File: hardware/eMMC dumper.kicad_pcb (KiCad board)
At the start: 2 copper layers, 67 x 43.2 mm, 52 parts, among them J1 Micro_SD_Card, J2 USB_B_Micro, J3 Conn_01x04, U1 F1C100s, U2 AMS1117-3.3, U3 TLV75512PDBV (WL9193S5-12), U4 EMMC04G-M627-A01

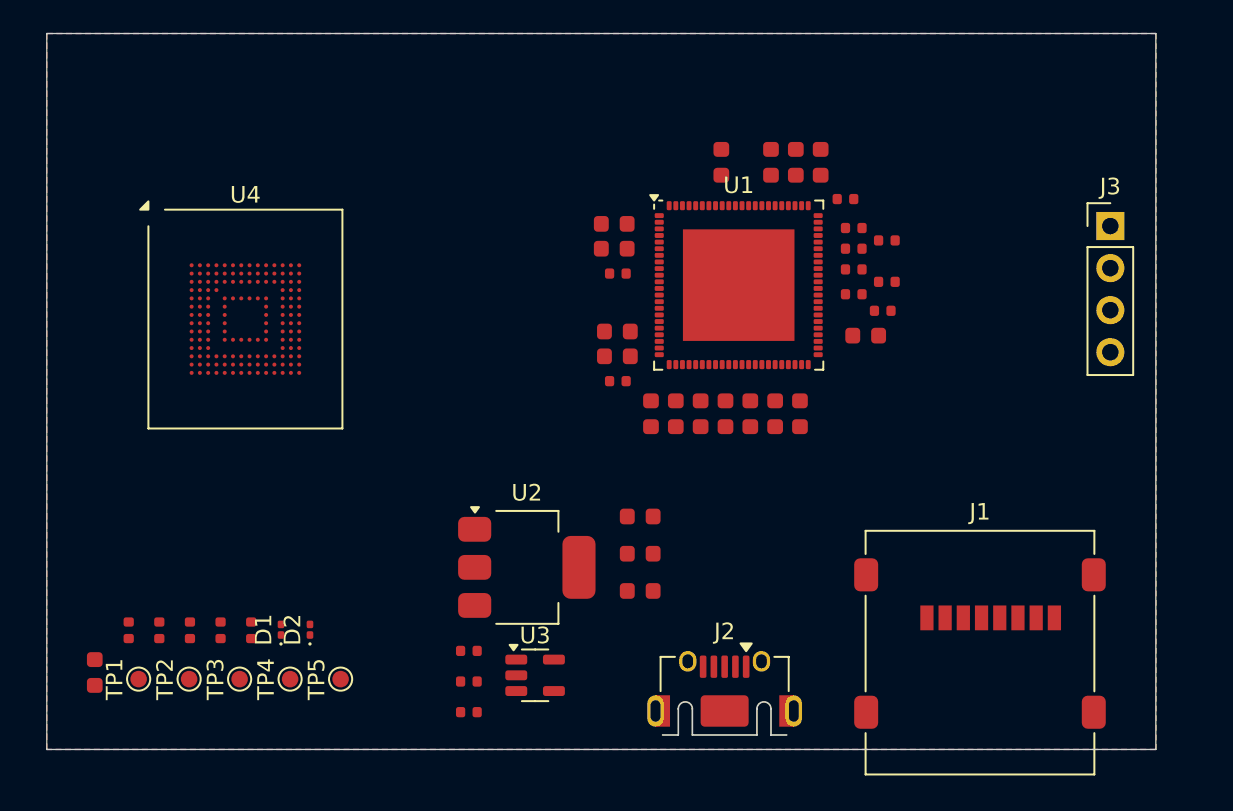
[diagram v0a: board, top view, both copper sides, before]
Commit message: PCB major changes
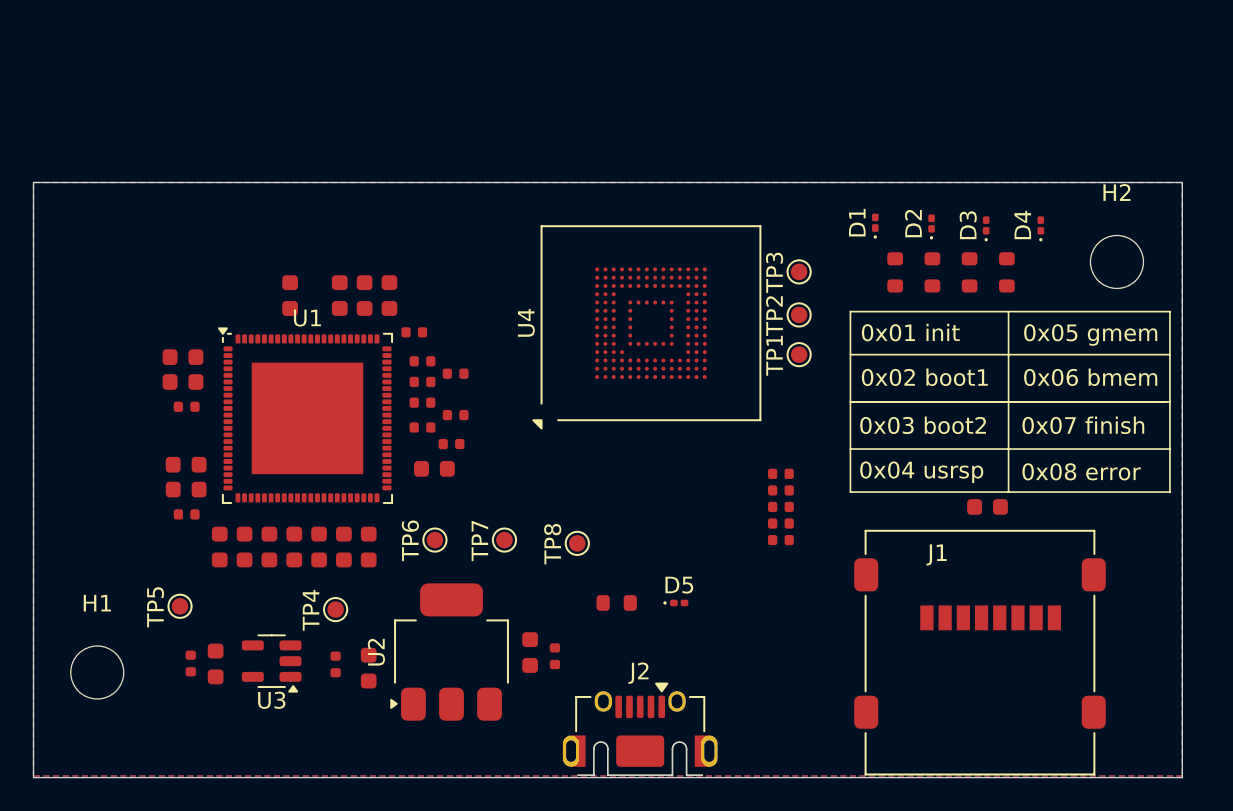
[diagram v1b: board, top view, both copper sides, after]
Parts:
- removed J3: Conn_01x04, Connector_PinHeader_2.54mm:PinHeader_1x04_P2.54mm_Vertical
- added D3: LED, LED_SMD:LED_0201_0603Metric, F.Cu at (182.5, 93.6)
- added D4: LED, LED_SMD:LED_0201_0603Metric, F.Cu at (185.8, 93.6)
- added D5: LED, LED_SMD:LED_0201_0603Metric, F.Cu at (164.0, 116.4)
- added H1: MountingHole, MountingHole:MountingHole_3.2mm_M3, F.Cu at (128.8, 120.6)
- added H2: MountingHole, MountingHole:MountingHole_3.2mm_M3, F.Cu at (190.4, 95.8)
- added R13: 1kΩ, PCM_JLCPCB:R_0603, F.Cu at (177.0, 96.4)
- added R14: 1kΩ, PCM_JLCPCB:R_0603, F.Cu at (179.2, 96.4)
- added R15: 1kΩ, PCM_JLCPCB:R_0603, F.Cu at (181.5, 96.4)
- added R16: 1kΩ, PCM_JLCPCB:R_0603, F.Cu at (183.8, 96.4)
- added R17: 1kΩ, PCM_JLCPCB:R_0603, F.Cu at (160.2, 116.4)
- added TP6: TestPoint, TestPoint:TestPoint_Pad_D1.0mm, F.Cu at (149.2, 112.6)
- added TP7: TestPoint, TestPoint:TestPoint_Pad_D1.0mm, F.Cu at (153.4, 112.6)
- added TP8: TestPoint, TestPoint:TestPoint_Pad_D1.0mm, F.Cu at (157.8, 112.8)
- moved C26 54.8 mm to (182.6, 110.6), turned to 0 degrees
- moved D2 44.9 mm to (179.2, 93.5)
- moved TP1 44.5 mm to (171.2, 101.4)
- moved D1 43.5 mm to (175.8, 93.4)
- moved TP2 42.9 mm to (171.2, 99.0)
- moved TP3 41.8 mm to (171.2, 96.4)
- moved R8 39.8 mm to (170.1, 112.6), turned to 0 degrees
- moved R9 38.1 mm to (170.1, 111.6), turned to 0 degrees
- moved R10 36.5 mm to (170.1, 110.6), turned to 0 degrees
- moved R11 34.9 mm to (170.1, 109.6), turned to 0 degrees
- moved R12 33.4 mm to (170.1, 108.6), turned to 0 degrees
- moved C10 27.3 mm to (144.9, 97.8)
- moved C11 27.3 mm to (146.4, 97.8)
- moved C12 27.3 mm to (134.2, 108.0)
- moved C13 27.3 mm to (149.2, 108.3)
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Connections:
- D1 pad 2: /Linux_core/LED_GRN -> /Linux_core/LED_1
- D2 pad 2: /Linux_core/LED_RED -> /Linux_core/LED_2
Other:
- board size 67 x 43.2 mm -> 69.4 x 36 mm
- board text added: "0x01 init"
- board text added: "0x02 boot1"
- board text added: "0x03 boot2"
- board text added: "0x04 usrsp"
- board text added: "0x05 gmem"
- board text added: "0x06 bmem"
- board text added: "0x07 finish"
- board text added: "0x08 error"
